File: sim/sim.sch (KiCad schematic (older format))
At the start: 4 parts

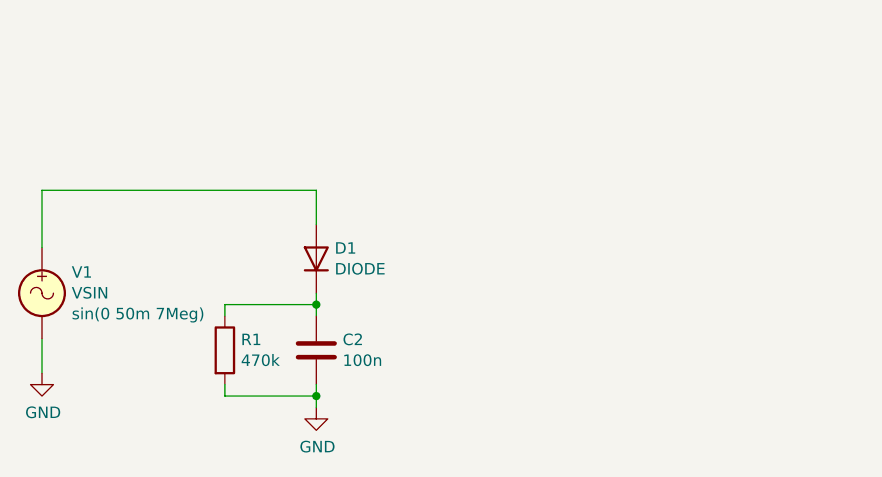
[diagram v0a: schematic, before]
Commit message: Final
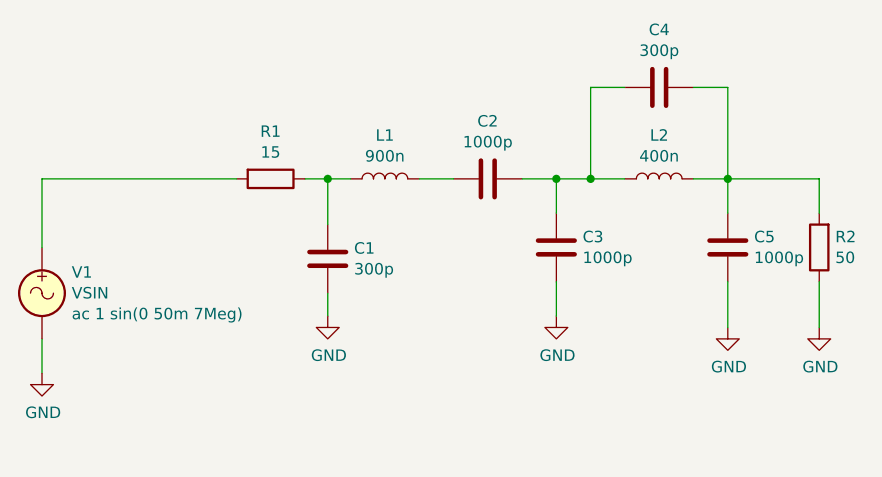
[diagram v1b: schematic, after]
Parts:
- removed D1: DIODE, symbol Simulation_SPICE:DIODE
- added C1, C4: 300p, symbol Device:C
- added C3, C5: 1000p, symbol Device:C
- added L1: 900n, symbol Device:L
- added L2: 400n, symbol Device:L
- added R2: 50, symbol Device:R
- C2: value 100n -> 1000p
- R1: value 470k -> 15
- V1: Spice_Model sin(0 50m 7Meg) -> ac 1 sin(0 50m 7Meg)
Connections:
- net GND: now also C1.2, C3.1, C5.1, R2.1; no longer C2.2, R1.2
- net at V1.1: now also R1.2
- net at R1.1: now also C1.1, L1.1; no longer C2.1
- new net: C2.2, L1.2
- new net: C2.1, C3.2, C4.1, L2.1
- new net: C4.2, C5.2, L2.2, R2.2
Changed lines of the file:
@@
 F 4 "Y" H 2850 3600 50  0001 L CNN "Spice_Netlist_Enabled"
 F 5 "V" H 2850 3600 50  0001 L CNN "Spice_Primitive"
-F 6 "sin(0 50m 7Meg)" H 2980 3509 50  0000 L CNN "Spice_Model"
+F 6 "ac 1 sin(0 50m 7Meg)" H 2980 3509 50  0000 L CNN "Spice_Model"
 	1    2850 3600
 	1    0    0    -1
@@
 	2850 3950 2850 3800
 $Comp
+L Device:R R1
+U 1 1 60CA45B4
+P 3850 3100
+F 0 "R1" V 3643 3100 50  0000 C CNN
+F 1 "15" V 3734 3100 50  0000 C CNN
+F 2 "" V 3780 3100 50  0001 C CNN
+F 3 "~" H 3850 3100 50  0001 C CNN
+	1    3850 3100
+	0    1    1    0
+$EndComp
+Wire Wire Line
+	2850 3100 3700 3100
+Wire Wire Line
+	2850 3100 2850 3400
+$Comp
+L Device:L L1
+U 1 1 60CA4CA0
+P 4350 3100
+F 0 "L1" V 4540 3100 50  0000 C CNN
+F 1 "900n" V 4449 3100 50  0000 C CNN
+F 2 "" H 4350 3100 50  0001 C CNN
+F 3 "~" H 4350 3100 50  0001 C CNN
+	1    4350 3100
+	0    -1   -1   0
+$EndComp
+$Comp
+L Device:C C1
+U 1 1 60CA62B7
+P 4100 3450
+F 0 "C1" H 4215 3496 50  0000 L CNN
+F 1 "300p" H 4215 3405 50  0000 L CNN
+F 2 "" H 4138 3300 50  0001 C CNN
+F 3 "~" H 4100 3450 50  0001 C CNN
+	1    4100 3450
+	1    0    0    -1
+$EndComp
+Wire Wire Line
+	4100 3300 4100 3100
+Wire Wire Line
+	4100 3100 4000 3100
+Wire Wire Line
+	4100 3100 4200 3100
+Connection ~ 4100 3100
+$Comp
+L power:GND #PWR02
+U 1 1 60CA6DCA
+P 4100 3700
+F 0 "#PWR02" H 4100 3450 50  0001 C CNN
+F 1 "GND" H 4105 3527 50  0000 C CNN
+F 2 "" H 4100 3700 50  0001 C CNN
+F 3 "" H 4100 3700 50  0001 C CNN
+	1    4100 3700
+	1    0    0    -1
+$EndComp
+Wire Wire Line
+	4100 3700 4100 3600
+$Comp
 L Device:C C2
-U 1 1 617893B8
-P 4050 3850
-F 0 "C2" H 4165 3896 50  0000 L CNN
-F 1 "100n" H 4165 3805 50  0000 L CNN
-F 2 "" H 4088 3700 50  0001 C CNN
-F 3 "~" H 4050 3850 50  0001 C CNN
-	1    4050 3850
-	1    0    0    -1
-$EndComp
-Wire Wire Line
-	4050 3700 4050 3650
-$Comp
-L power:GND #PWR02
-U 1 1 61789A47
-P 4050 4100
-F 0 "#PWR02" H 4050 3850 50  0001 C CNN
-F 1 "GND" H 4055 3927 50  0000 C CNN
-F 2 "" H 4050 4100 50  0001 C CNN
-F 3 "" H 4050 4100 50  0001 C CNN
-	1    4050 4100
-	1    0    0    -1
-$EndComp
-Wire Wire Line
-	4050 4100 4050 4050
-$Comp
-L Device:R R1
-U 1 1 6178A079
-P 3650 3850
-F 0 "R1" H 3720 3896 50  0000 L CNN
-F 1 "470k" H 3720 3805 50  0000 L CNN
-F 2 "" V 3580 3850 50  0001 C CNN
-F 3 "~" H 3650 3850 50  0001 C CNN
-	1    3650 3850
-	1    0    0    -1
-$EndComp
-Wire Wire Line
-	3650 3700 3650 3650
-Wire Wire Line
-	3650 3650 4050 3650
-Connection ~ 4050 3650
-Wire Wire Line
-	4050 3650 4050 3600
-Wire Wire Line
-	3650 4000 3650 4050
-Wire Wire Line
-	3650 4050 4050 4050
-Connection ~ 4050 4050
-Wire Wire Line
-	4050 4050 4050 4000
-Wire Wire Line
-	4050 3150 4050 3300
-Wire Wire Line
-	2850 3150 2850 3400
-$Comp
-L Simulation_SPICE:DIODE D1
-U 1 1 6179302F
-P 4050 3450
-F 0 "D1" V 4004 3530 50  0000 L CNN
-F 1 "DIODE" V 4095 3530 50  0000 L CNN
-F 2 "" H 4050 3450 50  0001 C CNN
-F 3 "~" H 4050 3450 50  0001 C CNN
-F 4 "Y" H 4050 3450 50  0001 L CNN "Spice_Netlist_Enabled"
-F 5 "D" H 4050 3450 50  0001 L CNN "Spice_Primitive"
-F 6 "BAT54" H 4050 3450 50  0001 C CNN "Spice_Model"
-F 7 "diode.lib" H 4050 3450 50  0001 C CNN "Spice_Lib_File"
-	1    4050 3450
+U 1 1 60CA7210
+P 4800 3100
+F 0 "C2" V 4548 3100 50  0000 C CNN
+F 1 "1000p" V 4639 3100 50  0000 C CNN
+F 2 "" H 4838 2950 50  0001 C CNN
+F 3 "~" H 4800 3100 50  0001 C CNN
+	1    4800 3100
 	0    1    1    0
 $EndComp
 Wire Wire Line
-	2850 3150 4050 3150
+	4650 3100 4500 3100
+$Comp
+L Device:C C3
+U 1 1 60CA7D4A
+P 5100 3400
+F 0 "C3" H 4985 3354 50  0000 R CNN
+F 1 "1000p" H 4985 3445 50  0000 R CNN
+F 2 "" H 5138 3250 50  0001 C CNN
+F 3 "~" H 5100 3400 50  0001 C CNN
+	1    5100 3400
+	-1   0    0    1
+$EndComp
+Wire Wire Line
+	4950 3100 5100 3100
+$Comp
+L power:GND #PWR03
+U 1 1 60CA8344
+P 5100 3700
+F 0 "#PWR03" H 5100 3450 50  0001 C CNN
+F 1 "GND" H 5105 3527 50  0000 C CNN
+F 2 "" H 5100 3700 50  0001 C CNN
+F 3 "" H 5100 3700 50  0001 C CNN
+	1    5100 3700
+	1    0    0    -1
+$EndComp
+Wire Wire Line
+	5100 3700 5100 3550
+$Comp
+L Device:L L2
+U 1 1 60CA8D04
+P 5550 3100
+F 0 "L2" V 5740 3100 50  0000 C CNN
+F 1 "400n" V 5649 3100 50  0000 C CNN
+F 2 "" H 5550 3100 50  0001 C CNN
+F 3 "~" H 5550 3100 50  0001 C CNN
+	1    5550 3100
+	0    -1   -1   0
+$EndComp
+Wire Wire Line
+	5400 3100 5250 3100
+Connection ~ 5100 3100
+$Comp
+L Device:C C5
+U 1 1 60CA93ED
+P 5850 3400
+F 0 "C5" H 5735 3354 50  0000 R CNN
+F 1 "1000p" H 5735 3445 50  0000 R CNN
+F 2 "" H 5888 3250 50  0001 C CNN
+F 3 "~" H 5850 3400 50  0001 C CNN
+	1    5850 3400
+	-1   0    0    1
+$EndComp
+$Comp
+L Device:C C4
+U 1 1 60CA9764
+P 5550 2700
+F 0 "C4" V 5802 2700 50  0000 C CNN
+F 1 "300p" V 5711 2700 50  0000 C CNN
+F 2 "" H 5588 2550 50  0001 C CNN
+F 3 "~" H 5550 2700 50  0001 C CNN
+	1    5550 2700
+	0    -1   -1   0
+$EndComp
+Wire Wire Line
+	5400 2700 5250 2700
+Wire Wire Line
+	5250 2700 5250 3100
+Wire Wire Line
+	5100 3100 5100 3250
+Connection ~ 5250 3100
+Wire Wire Line
+	5250 3100 5100 3100
+Wire Wire Line
+	5700 2700 5850 2700
+Wire Wire Line
+	5850 2700 5850 3100
+Wire Wire Line
+	5850 3100 5700 3100
+Wire Wire Line
+	5850 3100 5850 3250
+Connection ~ 5850 3100
+$Comp
+L power:GND #PWR04
+U 1 1 60CAA65B
+P 5850 3750
+F 0 "#PWR04" H 5850 3500 50  0001 C CNN
+F 1 "GND" H 5855 3577 50  0000 C CNN
+F 2 "" H 5850 3750 50  0001 C CNN
+F 3 "" H 5850 3750 50  0001 C CNN
+	1    5850 3750
+	1    0    0    -1
+$EndComp
+Wire Wire Line
+	5850 3750 5850 3550
+$Comp
+L Device:R R2
+U 1 1 60CAAD0B
+P 6250 3400
+F 0 "R2" H 6180 3354 50  0000 R CNN
+F 1 "50" H 6180 3445 50  0000 R CNN
+F 2 "" V 6180 3400 50  0001 C CNN
+F 3 "~" H 6250 3400 50  0001 C CNN
+	1    6250 3400
+	-1   0    0    1
+$EndComp
+Wire Wire Line
+	5850 3100 6250 3100
+Wire Wire Line
+	6250 3100 6250 3250
+$Comp
+L power:GND #PWR05
+U 1 1 60CAB4F6
+P 6250 3750
+F 0 "#PWR05" H 6250 3500 50  0001 C CNN
+F 1 "GND" H 6255 3577 50  0000 C CNN
+F 2 "" H 6250 3750 50  0001 C CNN
+F 3 "" H 6250 3750 50  0001 C CNN
+	1    6250 3750
+	1    0    0    -1
+$EndComp
+Wire Wire Line
+	6250 3750 6250 3550
 $EndSCHEMATC
